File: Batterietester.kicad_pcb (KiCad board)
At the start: 2 copper layers, 15 parts, among them J1 Load, J2 Power, SW1 SW_Push, SW2 SW_Push, U1 LM3914

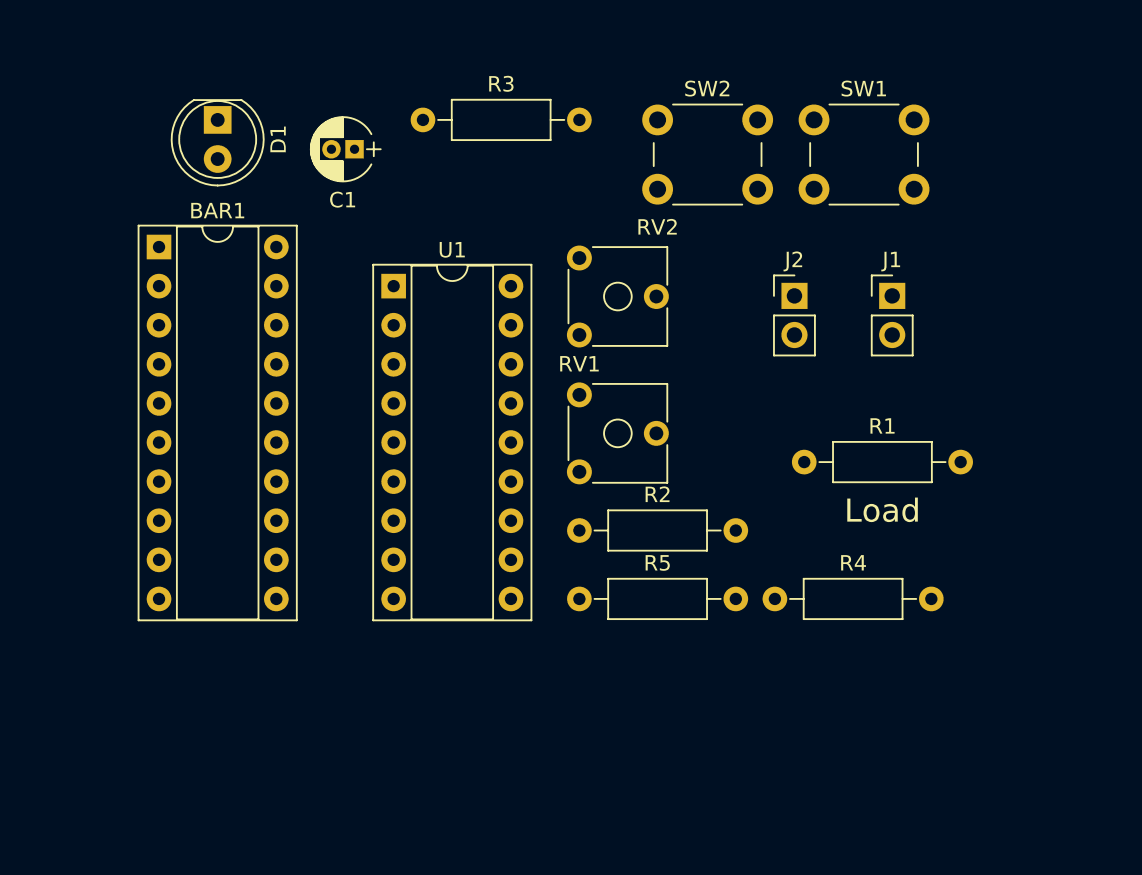
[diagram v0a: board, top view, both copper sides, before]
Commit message: Board design
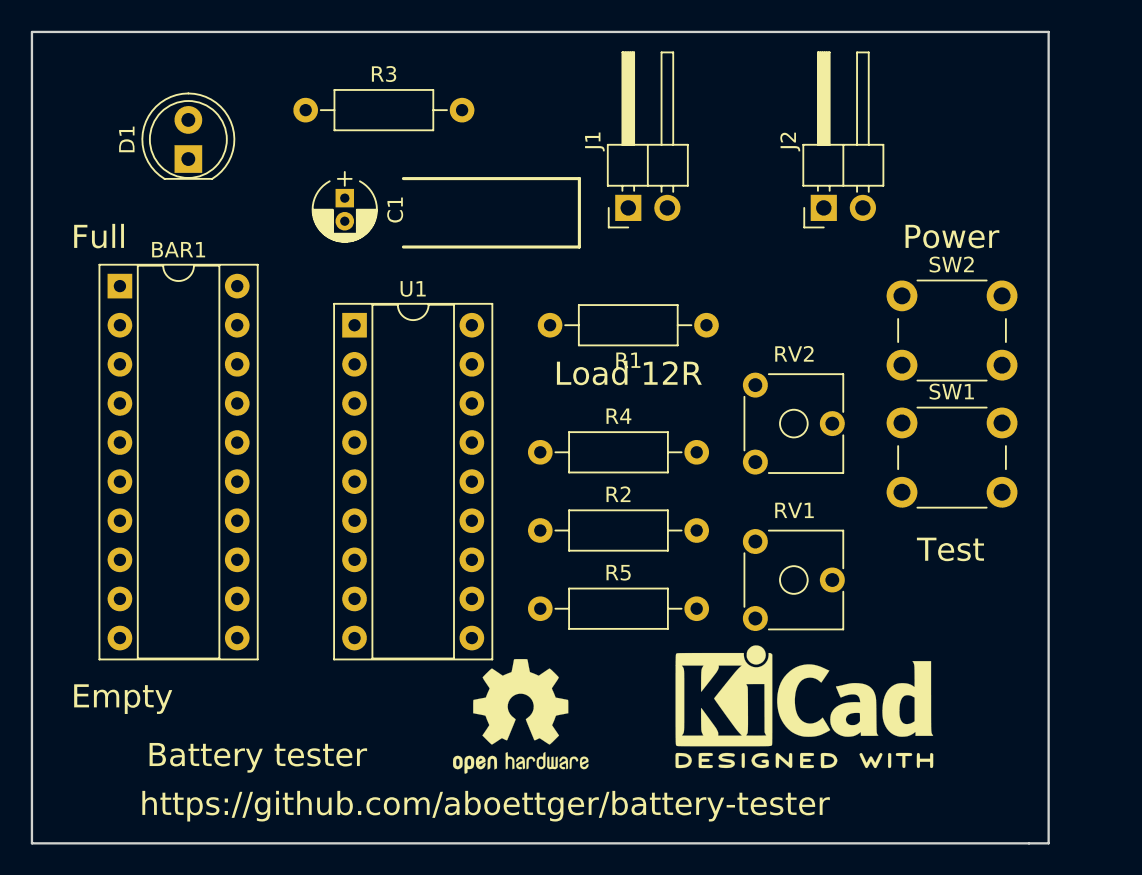
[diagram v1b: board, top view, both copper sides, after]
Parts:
- added REF***: KiCad-Logo2_8mm_SilkScreen, Symbols:KiCad-Logo2_8mm_SilkScreen, F.Cu at (148.6, 114.9)
- added REF***: OSHW-Logo2_9.8x8mm_SilkScreen, Symbols:OSHW-Logo2_9.8x8mm_SilkScreen, F.Cu at (130.2, 115.6)
- J1, J2: footprint Pin_Headers:Pin_Header_Straight_1x02_Pitch2.54mm -> Pin_Headers:Pin_Header_Angled_1x02_Pitch2.54mm
- moved SW1 20.5 mm to (154.9, 96.5)
- moved SW2 19.6 mm to (154.9, 88.3)
- moved J1 18.1 mm to (137.2, 82.5), turned to 90 degrees
- moved R4 18.0 mm to (131.4, 98.4)
- moved RV1 14.9 mm to (145.4, 109.2)
- moved RV2 14.1 mm to (145.4, 99.1)
- moved R1 10.9 mm to (142.2, 90.2), turned to 180 degrees
- moved R3 7.65 mm to (116.2, 76.2)
- moved J2 6.02 mm to (149.9, 82.5), turned to 90 degrees
- moved U1 3.59 mm to (119.4, 90.2)
- moved BAR1 3.59 mm to (104.1, 87.6)
- moved C1 3.24 mm to (118.7, 81.9), turned to 270 degrees
- moved D1 3.18 mm to (108.6, 79.4), turned to 90 degrees
- moved R5 2.62 mm to (131.4, 108.6)
- moved R2 2.54 mm to (131.4, 103.5)
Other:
- board outline added: 66 x 52.7 mm
- board text added: "Battery tester"
- board text added: "Empty"
- board text added: "Full"
- board text added: "Load 12R"
- board text added: "Power"
- board text added: "Test"
- board text added: "https://github.com/aboettger/battery-tester"
- board text removed: "Load"
